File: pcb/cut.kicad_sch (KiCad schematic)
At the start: 34 parts, among them J4 RJ12, J5 RJ12, J6 Conn_01x02, J7 Conn_01x02, K1 AZ850-5, K2 AZ850-5, Q1 2N7002, Q2 2N7002, U5 PC817, U6 PC817

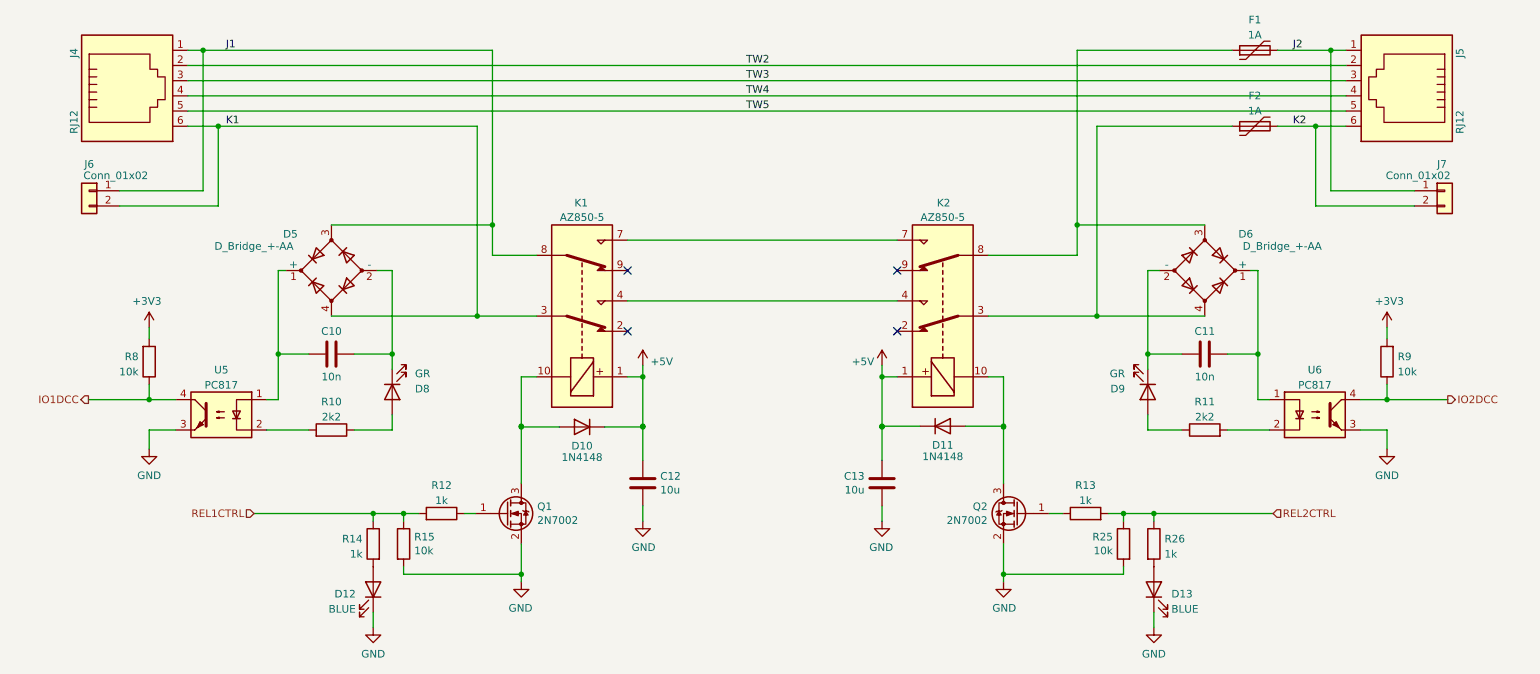
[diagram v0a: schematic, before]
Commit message: Use dicrete schottky diodes for dcc rectifiers.
Schottky diodes do not cause short-time shortcuts.
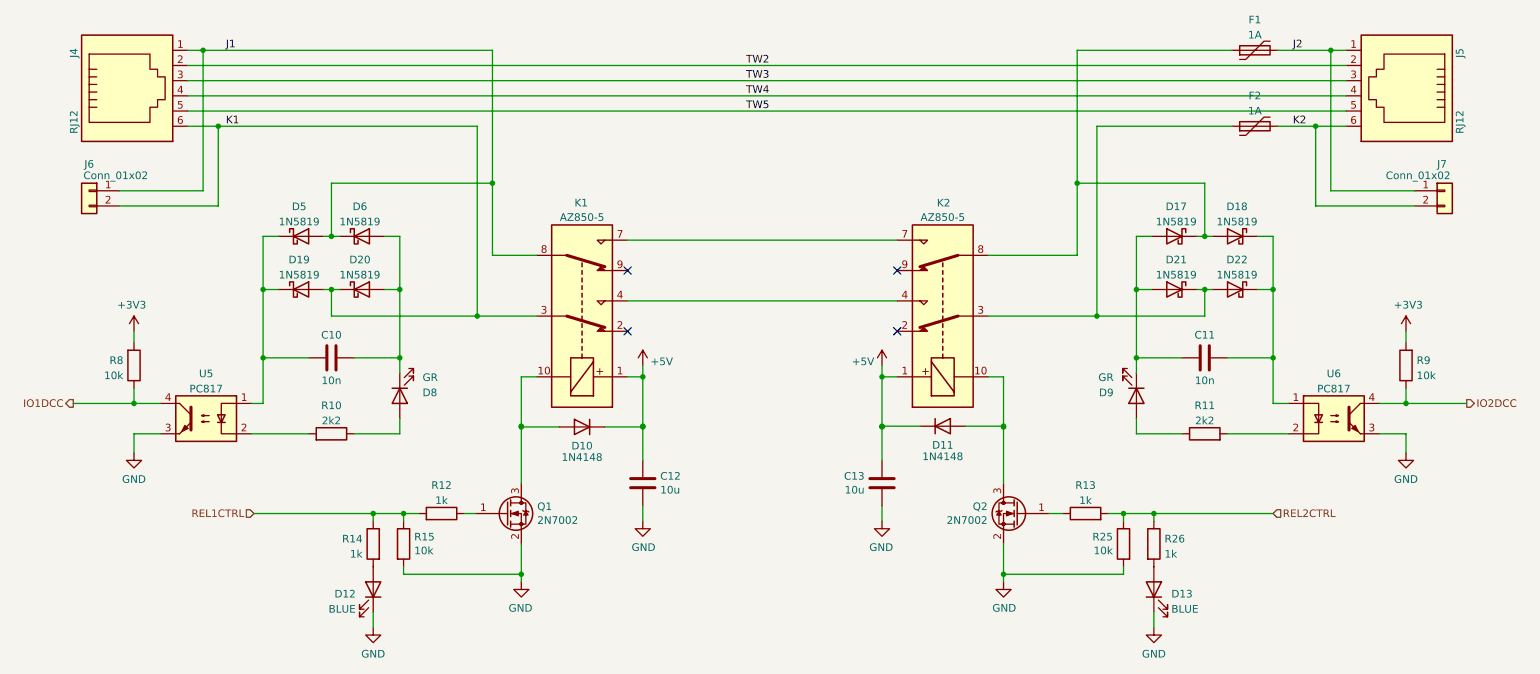
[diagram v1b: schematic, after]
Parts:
- removed D5, D6: D_Bridge_+-AA, Rectifiers:S250, symbol Device:D_Bridge_+-AA
- added D17, D18, D19, D20, D21, D22, D5, D6: 1N5819, Diode_SMD:D_SOD-123, symbol Diode:1N5819
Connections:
- net J1: now also D5.2 (A), D6.1 (K)
- net K1: now also D19.2 (A), D20.1 (K)
- net at C11.1, D9.1 (K): now also D17.2 (A), D21.2 (A)
- net at F1.1, K2.8: now also D17.1 (K), D18.2 (A)
- net at C10.1, U5.1: now also D19.1 (K), D5.1 (K)
- net at C10.2, D8.1 (K): now also D20.2 (A), D6.2 (A)
- net at F2.1, K2.3: now also D21.1 (K), D22.2 (A)
- net at C11.2, U6.1: now also D18.1 (K), D22.1 (K)
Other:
- moved on the sheet: C10, C11, D8, D9, R10, R11, R8, R9, U5, U6
